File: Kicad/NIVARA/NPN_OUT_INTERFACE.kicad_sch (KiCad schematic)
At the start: 8 parts, among them Q1 NCV8402xST, Q3 NCV8402xST, U12 LTV-357T, U5 LTV-357T

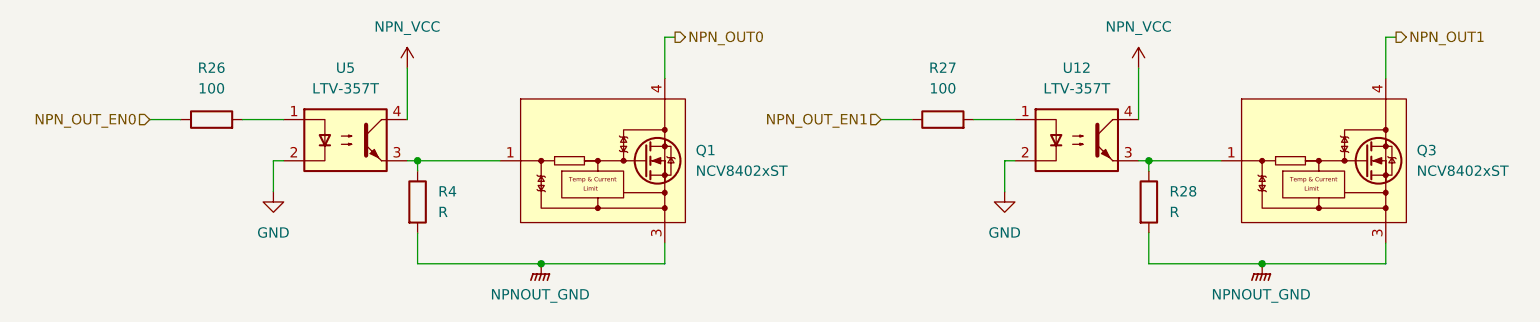
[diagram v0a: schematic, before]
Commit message: FULL SCHEMATIC!!111!!!
Dik
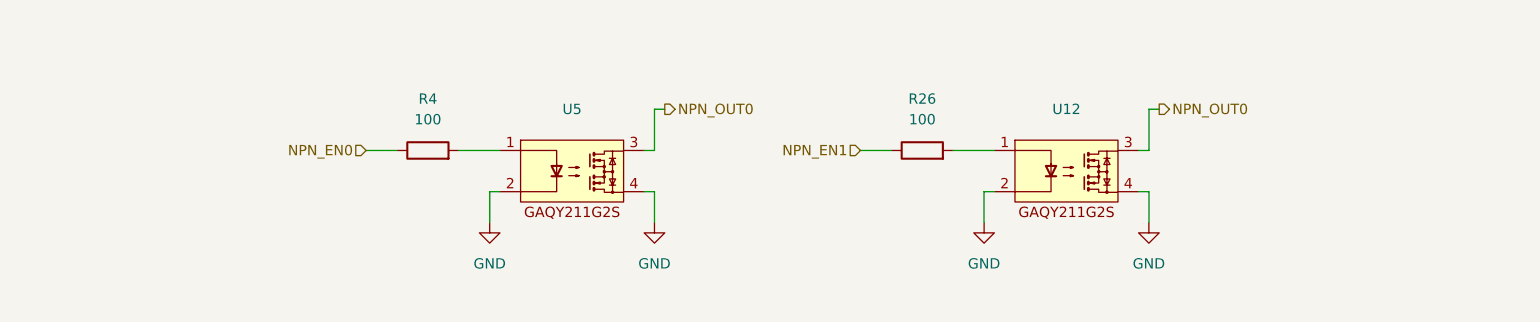
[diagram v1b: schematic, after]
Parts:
- removed Q1, Q3: NCV8402xST, Package_TO_SOT_SMD:SOT-223, symbol Driver_FET:NCV8402xST
- removed R27: 100, symbol Device:R
- removed R28: R, symbol Device:R
- removed U12, U5: LTV-357T, Package_SO:SO-4_4.4x3.6mm_P2.54mm, symbol Isolator:LTV-357T
- added U12, U5: ~, Package_SO:SO-4_4.4x4.3mm_P2.54mm, symbol Riqi_Parts:GAQY211G2S
- R4: value R -> 100
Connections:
- net GND: now also U12.2, U12.4, U5.2, U5.4
- net NPN_OUT0: now also U12.3, U5.3
- net at R26.2: now also U12.1
- net NPN_EN0: now reaches R4.1
- net NPNOUT_GND: no longer names the net of R4.2
- net NPNOUT_GND: now also U5.1
- net NPN_OUT_EN0 renamed NPN_EN1

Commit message: Debí de enrutar antes :C
tengo sueño
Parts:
- R26, R4: footprint (none) -> Resistor_SMD:R_0603_1608Metric
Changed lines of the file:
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@@
 			)
 		)
-		(property "Footprint" ""
+		(property "Footprint" "Resistor_SMD:R_0603_1608Metric"
 			(at 172.72 89.408 90)
 			(effects
@@
 			)
 		)
-		(property "Footprint" ""
+		(property "Footprint" "Resistor_SMD:R_0603_1608Metric"
 			(at 111.76 89.408 90)
 			(effects
